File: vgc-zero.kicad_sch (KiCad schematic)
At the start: 22 parts, among them J1 Conn_01x06_Pin, J2 Conn_01x06_Pin, J3 Conn_01x06_Pin, SW1 SW_Push, SW10 SW_Push, SW11 SW_SPDT, SW2 SW_Push, SW3 SW_Push, SW4 SW_Push, SW5 SW_Push, SW6 SW_Push, SW7 SW_Push, SW8 SW_Push, SW9 SW_Push

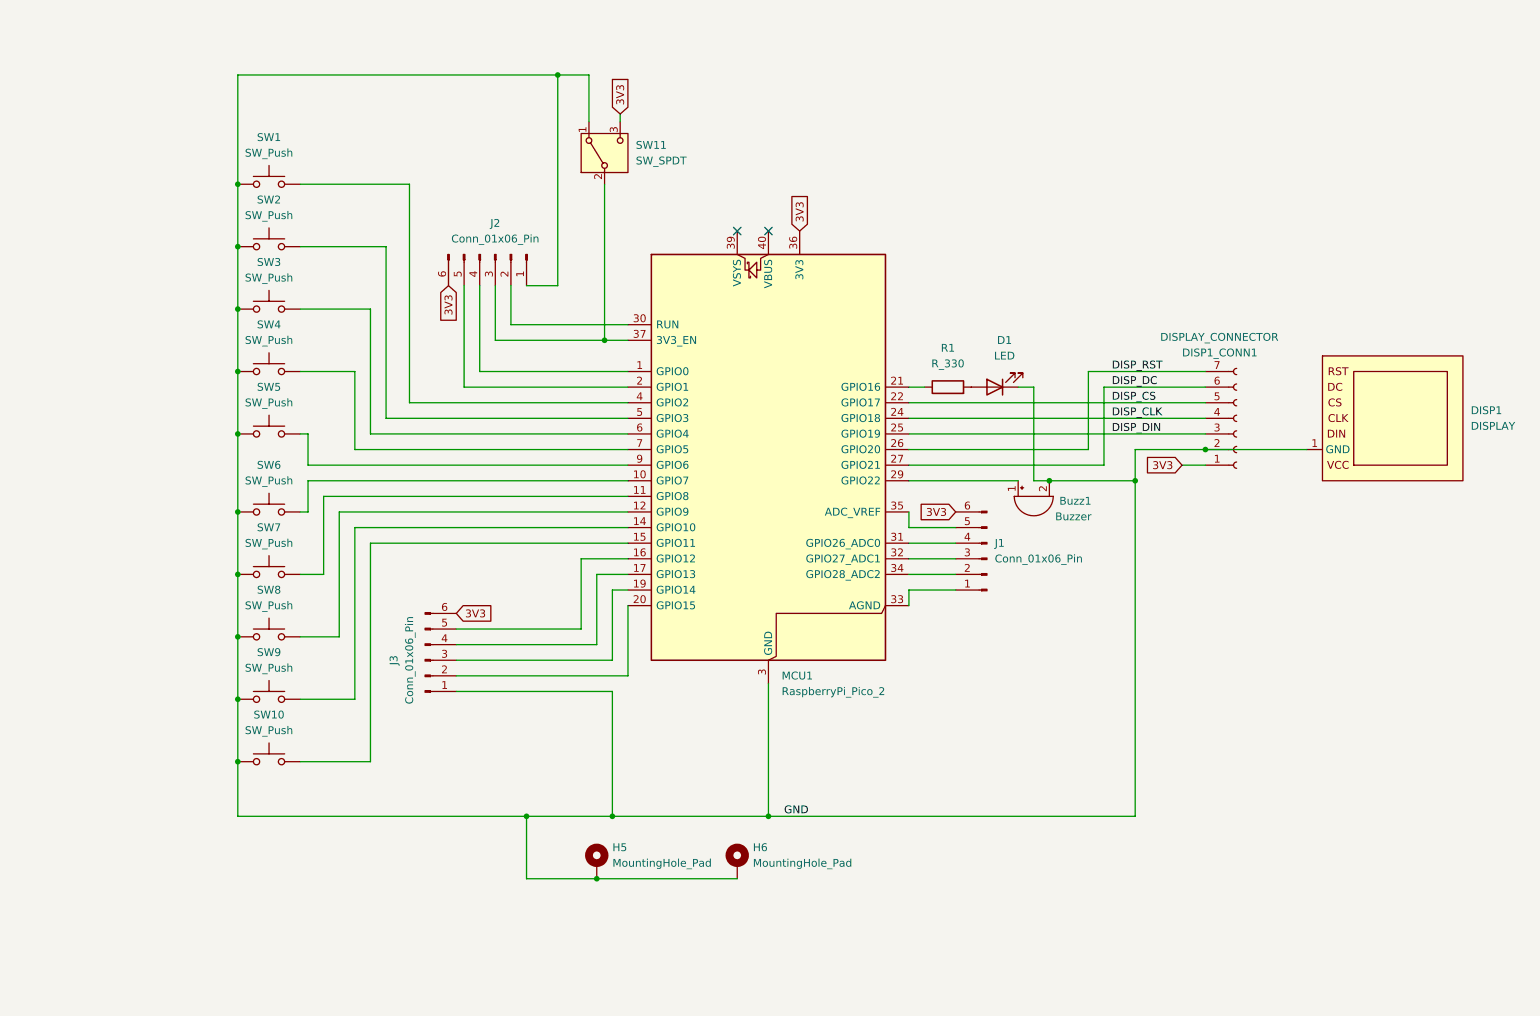
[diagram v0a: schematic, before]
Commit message: new version changes
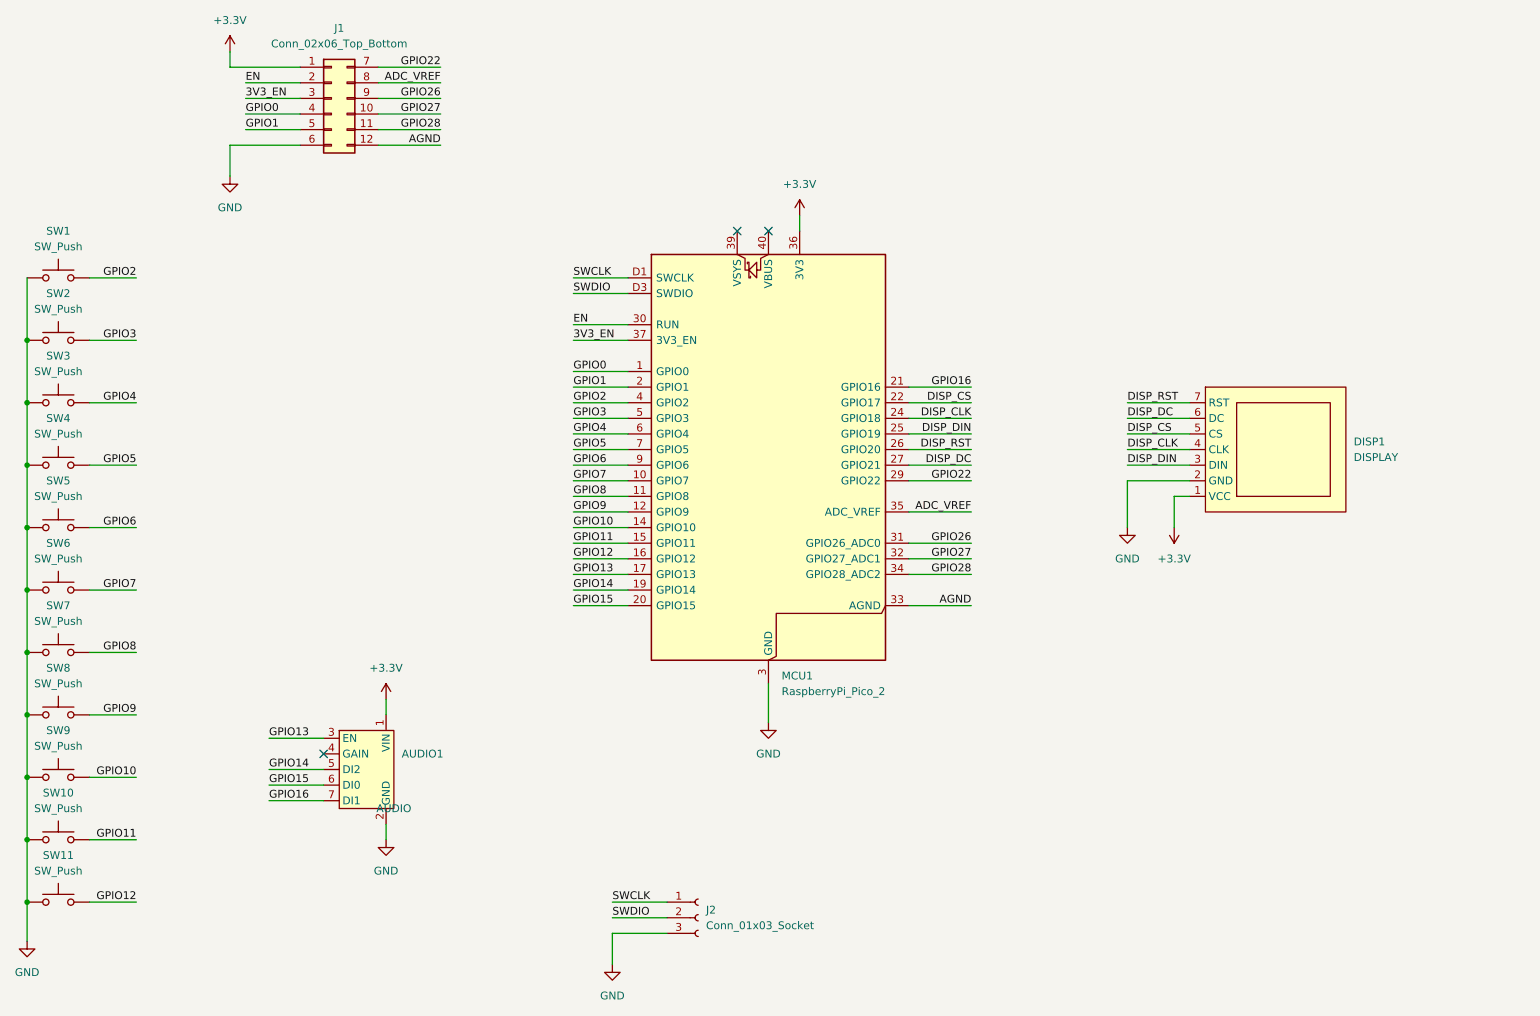
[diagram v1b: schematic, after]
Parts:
- removed Buzz1: Buzzer, Buzzer_Beeper:Buzzer_12x9.5RM7.6, symbol Device:Buzzer
- removed D1: LED, LED_SMD:LED_1210_3225Metric_Pad1.42x2.65mm_HandSolder, symbol Device:LED
- removed DISP1_CONN1: DISPLAY_CONNECTOR, Connector_JST:JST_PH_S7B-PH-K_1x07_P2.00mm_Horizontal, symbol Connector:Conn_01x07_Socket
- removed H5, H6: MountingHole_Pad, MountingHole:MountingHole_2.2mm_M2_Pad, symbol Mechanical:MountingHole_Pad
- removed J1, J2, J3: Conn_01x06_Pin, Connector_PinHeader_2.54mm:PinHeader_1x06_P2.54mm_Horizontal, symbol Connector:Conn_01x06_Pin
- removed R1: R_330, Resistor_THT:R_Axial_DIN0204_L3.6mm_D1.6mm_P5.08mm_Horizontal, symbol Device:R
- removed SW11: SW_SPDT, Button_Switch_THT:SW_Slide_SPDT_Angled_CK_OS102011MA1Q, symbol Switch:SW_SPDT
- added AUDIO1: AUDIO, vgc-zero-footprints:Untitled, symbol vgc-zero-symbols:AudioModule
- added J1: Conn_02x06_Top_Bottom, Connector_PinSocket_2.54mm:PinSocket_2x05_P2.54mm_Horizontal, symbol Connector_Generic:Conn_02x06_Top_Bottom
- added J2: Conn_01x03_Socket, Connector_JST:JST_SH_SM03B-SRSS-TB_1x03-1MP_P1.00mm_Horizontal, symbol Connector:Conn_01x03_Socket
- added SW11: SW_Push, Button_Switch_THT:SW_Tactile_SPST_Angled_PTS645Vx58-2LFS, symbol Switch:SW_Push
- MCU1: footprint Module:RaspberryPi_Pico_Common_THT -> Module:RaspberryPi_Pico_SMD_HandSolder; symbol MCU_Module:RaspberryPi_Pico -> MCU_Module:RaspberryPi_Pico_Debug
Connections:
- net DISP_CLK: now also DISP1.4 (CLK)
- net DISP_CS: now also DISP1.5 (CS)
- net DISP_DC: now also DISP1.6 (DC)
- net DISP_DIN: now also DISP1.3 (DIN)
- net DISP_RST: now also DISP1.7 (RST)
- net GND: now also DISP1.2 (GND), MCU1.D2 (GND), AUDIO1.2 (GND), J1.6 (Pin_6), J2.3 (Pin_3), SW11.1; no longer DISP1.1 (GND)
- net GPIO0: now reaches MCU1.1 (GPIO0)
- net GPIO0: now also J1.4 (Pin_4)
- net GPIO7: now reaches MCU1.10 (GPIO7), SW6.2
- net GPIO8: now reaches MCU1.11 (GPIO8), SW7.2
- net GPIO9: now reaches MCU1.12 (GPIO9), SW8.2
- net GPIO10: now reaches MCU1.14 (GPIO10), SW9.2
- net GPIO11: now reaches MCU1.15 (GPIO11), SW10.2
- net GPIO12: now reaches MCU1.16 (GPIO12)
- net GPIO12: now also SW11.2
- net GPIO13: now reaches MCU1.17 (GPIO13)
- net GPIO13: now also AUDIO1.3 (EN)
- net GPIO14: now reaches MCU1.19 (GPIO14)
- net GPIO14: now also AUDIO1.5 (DI2)
- net GPIO1: now reaches MCU1.2 (GPIO1)
- net GPIO1: now also J1.5 (Pin_5)
- net GPIO15: now reaches MCU1.20 (GPIO15)
- net GPIO15: now also AUDIO1.6 (DI0)
- net GPIO16: now reaches MCU1.21 (GPIO16)
- net GPIO16: now also AUDIO1.7 (DI1)
- net GPIO22: now reaches MCU1.29 (GPIO22)
- net GPIO22: now also J1.7 (Pin_7)
- net EN: now reaches MCU1.30 (RUN)
- net EN: now also J1.2 (Pin_2)
- net GPIO26: now reaches MCU1.31 (GPIO26_ADC0)
- net GPIO26: now also J1.9 (Pin_9)
- net GPIO27: now reaches MCU1.32 (GPIO27_ADC1)
- net GPIO27: now also J1.10 (Pin_10)
- net AGND: now reaches MCU1.33 (AGND)
- net AGND: now also J1.12 (Pin_12)
- net GPIO28: now reaches MCU1.34 (GPIO28_ADC2)
- net GPIO28: now also J1.11 (Pin_11)
- net ADC_VREF: now reaches MCU1.35 (ADC_VREF)
- net ADC_VREF: now also J1.8 (Pin_8)
- net 3V3_EN: now reaches MCU1.37 (3V3_EN)
- net 3V3_EN: now also J1.3 (Pin_3)
- net GPIO2: now reaches MCU1.4 (GPIO2), SW1.2
- net GPIO3: now reaches MCU1.5 (GPIO3), SW2.2
- net GPIO4: now reaches MCU1.6 (GPIO4), SW3.2
- net GPIO5: now reaches MCU1.7 (GPIO5), SW4.2
- net GPIO6: now reaches MCU1.9 (GPIO6), SW5.2
- net 3V3 renamed +3.3V
- net +3.3V: now also DISP1.1 (VCC), AUDIO1.1 (VIN), J1.1 (Pin_1)
- new net SWCLK: J2.1 (Pin_1), MCU1.D1 (SWCLK)
- new net SWDIO: J2.2 (Pin_2), MCU1.D3 (SWDIO)
- no-connect marks 2 -> 3
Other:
- moved on the sheet: SW1, SW10, SW2, SW3, SW4, SW5, SW6, SW7, SW8, SW9
